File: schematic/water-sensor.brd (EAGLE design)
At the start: 81 x 58.4 mm, 8 parts, among them X1 XRJK-S-01-6-4-0-9M2

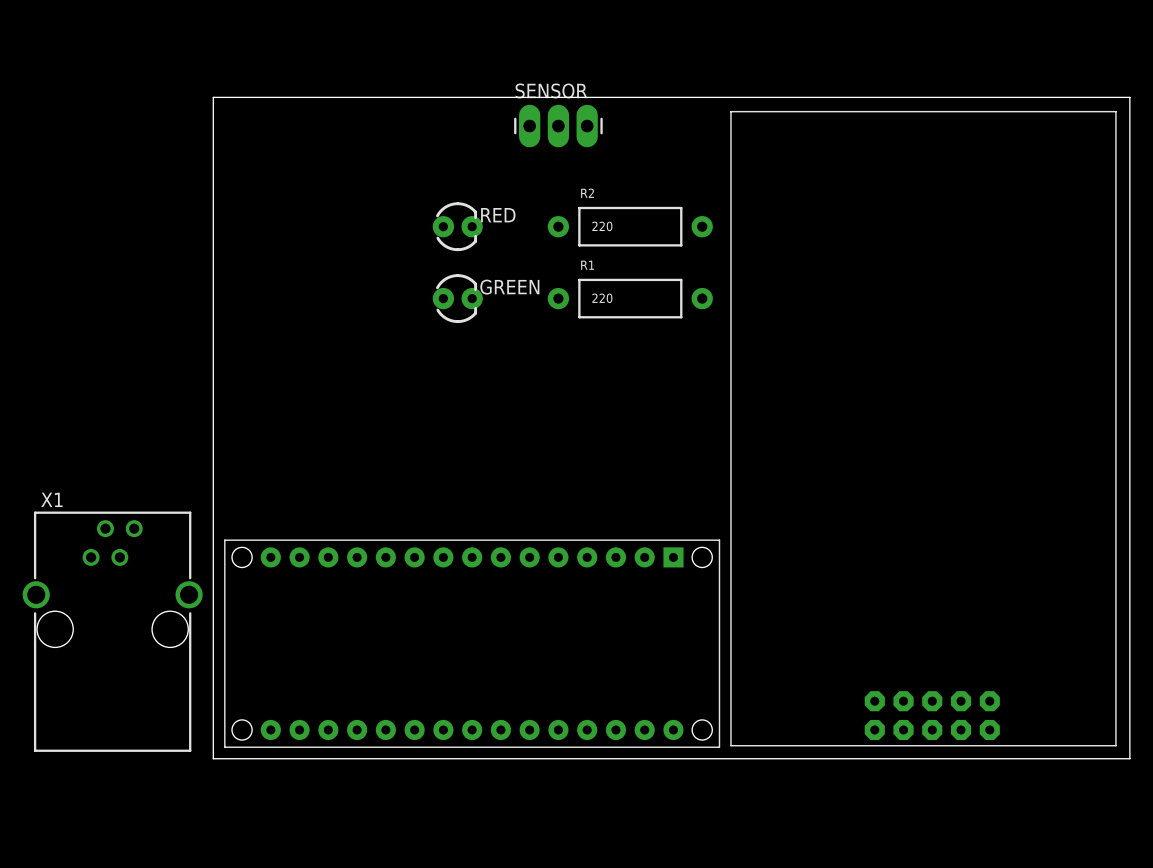
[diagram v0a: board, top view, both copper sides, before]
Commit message: water sensor
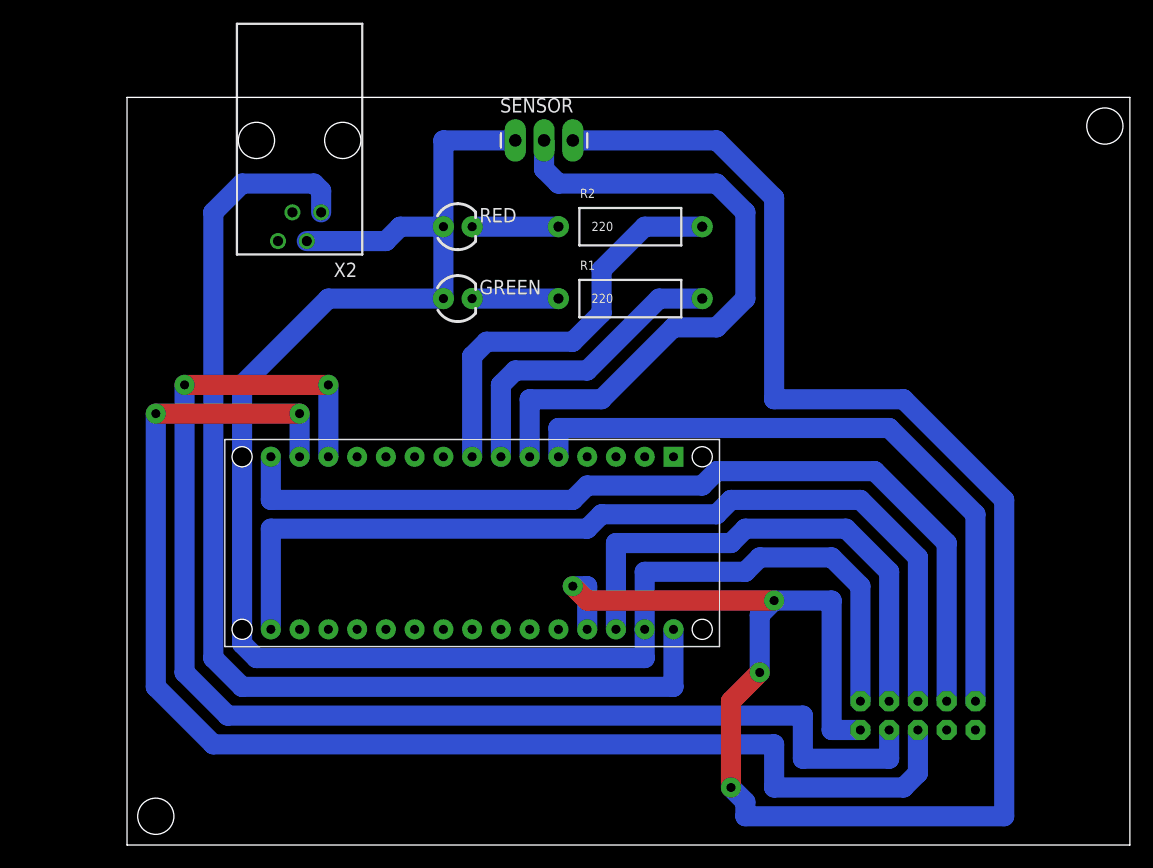
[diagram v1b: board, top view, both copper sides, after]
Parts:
- removed X1: XRJK-S-01-6-4-0-9M2, con-xmultiple:XRJK-S-01-6-4-0-9M2
- added X2: 14867, con-4ucon:14867
- moved U$2 34.3 mm to (99.1, 57.1), flipped to the bottom
- moved U$1 8.89 mm to (62.2, 26.7)
- moved SENSOR 1.80 mm to (45.7, 54.6)
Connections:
- net 5V: now also U$2.VCC
- net D10: now also U$2.CS
- net D11: now also U$2.SI
- net D12: now also U$2.SO
- net D13: now also U$2.SCK
- net D2: now also U$2.INT
- net GND: now also U$2.GND, X2.2
- net RESET: now also U$2.RESET
- net VIN: now also X2.1
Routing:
- net 5V: track 0.00 -> 176.1 mm, vias 0 -> 4
- net GND: track 0.00 -> 151.2 mm
- net D11: track 0.00 -> 118.2 mm, vias 0 -> 2
- net D10: track 0.00 -> 114.6 mm, vias 0 -> 2
- net VIN: track 0.00 -> 98.9 mm
- net D13: track 0.00 -> 81.9 mm
- net D12: track 0.00 -> 81.2 mm
- net D2: track 0.00 -> 59.0 mm
- net D3: track 0.00 -> 57.3 mm
- net RESET: track 0.00 -> 45.3 mm
- net D5: track 0.00 -> 36.2 mm
- net D4: track 0.00 -> 27.3 mm
- net N$2: track 0.00 -> 7.62 mm
- net N$1: track 0.00 -> 7.62 mm
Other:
- board size 81 x 58.4 mm -> 88.6 x 66 mm
